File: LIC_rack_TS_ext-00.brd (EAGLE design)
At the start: 72 x 52 mm, 31 parts, among them K1 FINDER 40.52.9.024.0000, X1 22-23-2041, X10 WAGO236-401/2, X11 22-23-2041, X12 22-23-2041, X13 22-23-2021, X14 22-23-2021, X15 22-23-2021, X2 22-23-2041, X3 22-23-2041, X4 22-23-2041, X5 22-23-2021, X6 22-23-2021, X7 22-23-2021, X8 22-23-2021, X9 WAGO236-401/2

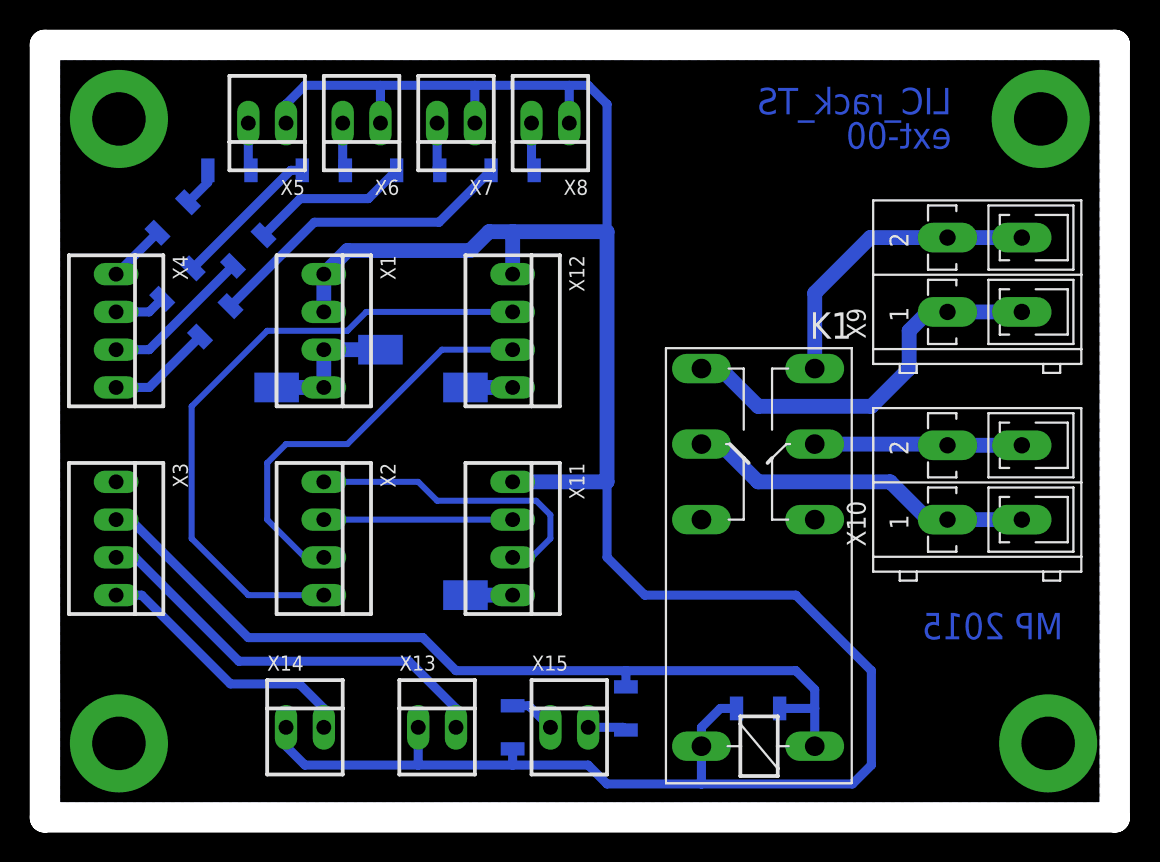
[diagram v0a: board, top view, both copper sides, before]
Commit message: v.1.0
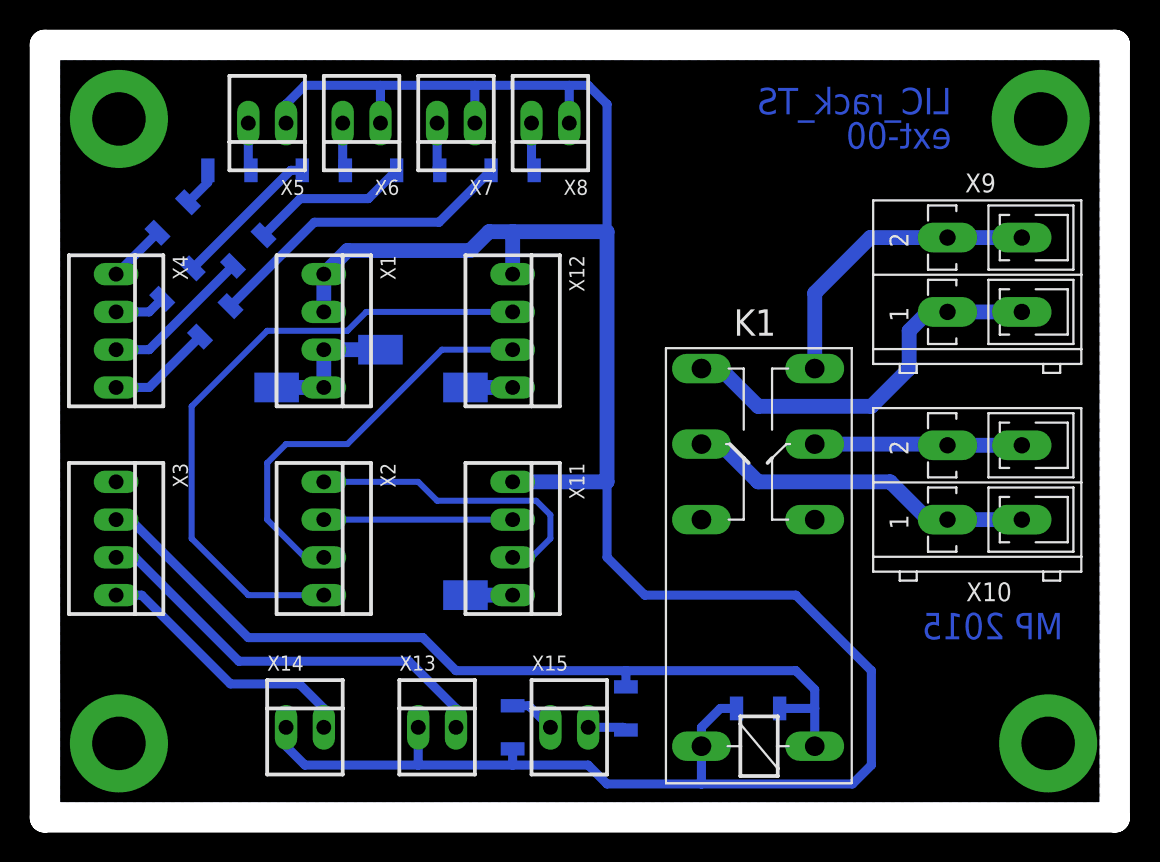
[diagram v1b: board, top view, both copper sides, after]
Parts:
- added U$2: (no value), frames:A4L-LOC
- X1: value 22-23-2041 -> Supply
- X10: value WAGO236-401/2 -> High Voltage Supply - N
- X11: value 22-23-2041 -> BronkHorst - A
- X12: value 22-23-2041 -> BronkHorst - B
- X13: value 22-23-2021 -> El.Mag - A
- X14: value 22-23-2021 -> El.Mag - B
- X15: value 22-23-2021 -> Rot Vyveva - Rele
- X2: value 22-23-2041 -> BronkHorst IN
- X3: value 22-23-2041 -> ROT-EM A a B
- X4: value 22-23-2041 -> LED_IN
- X5: value 22-23-2021 -> LED_OUT_1
- X6: value 22-23-2021 -> LED_OUT_2
- X7: value 22-23-2021 -> LED_OUT_3
- X8: value 22-23-2021 -> LED_OUT_4
- X9: value WAGO236-401/2 -> High Voltage Supply - L
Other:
- board text added: "00"
- board text added: "Top view"
